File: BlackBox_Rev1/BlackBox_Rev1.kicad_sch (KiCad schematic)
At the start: 15 parts

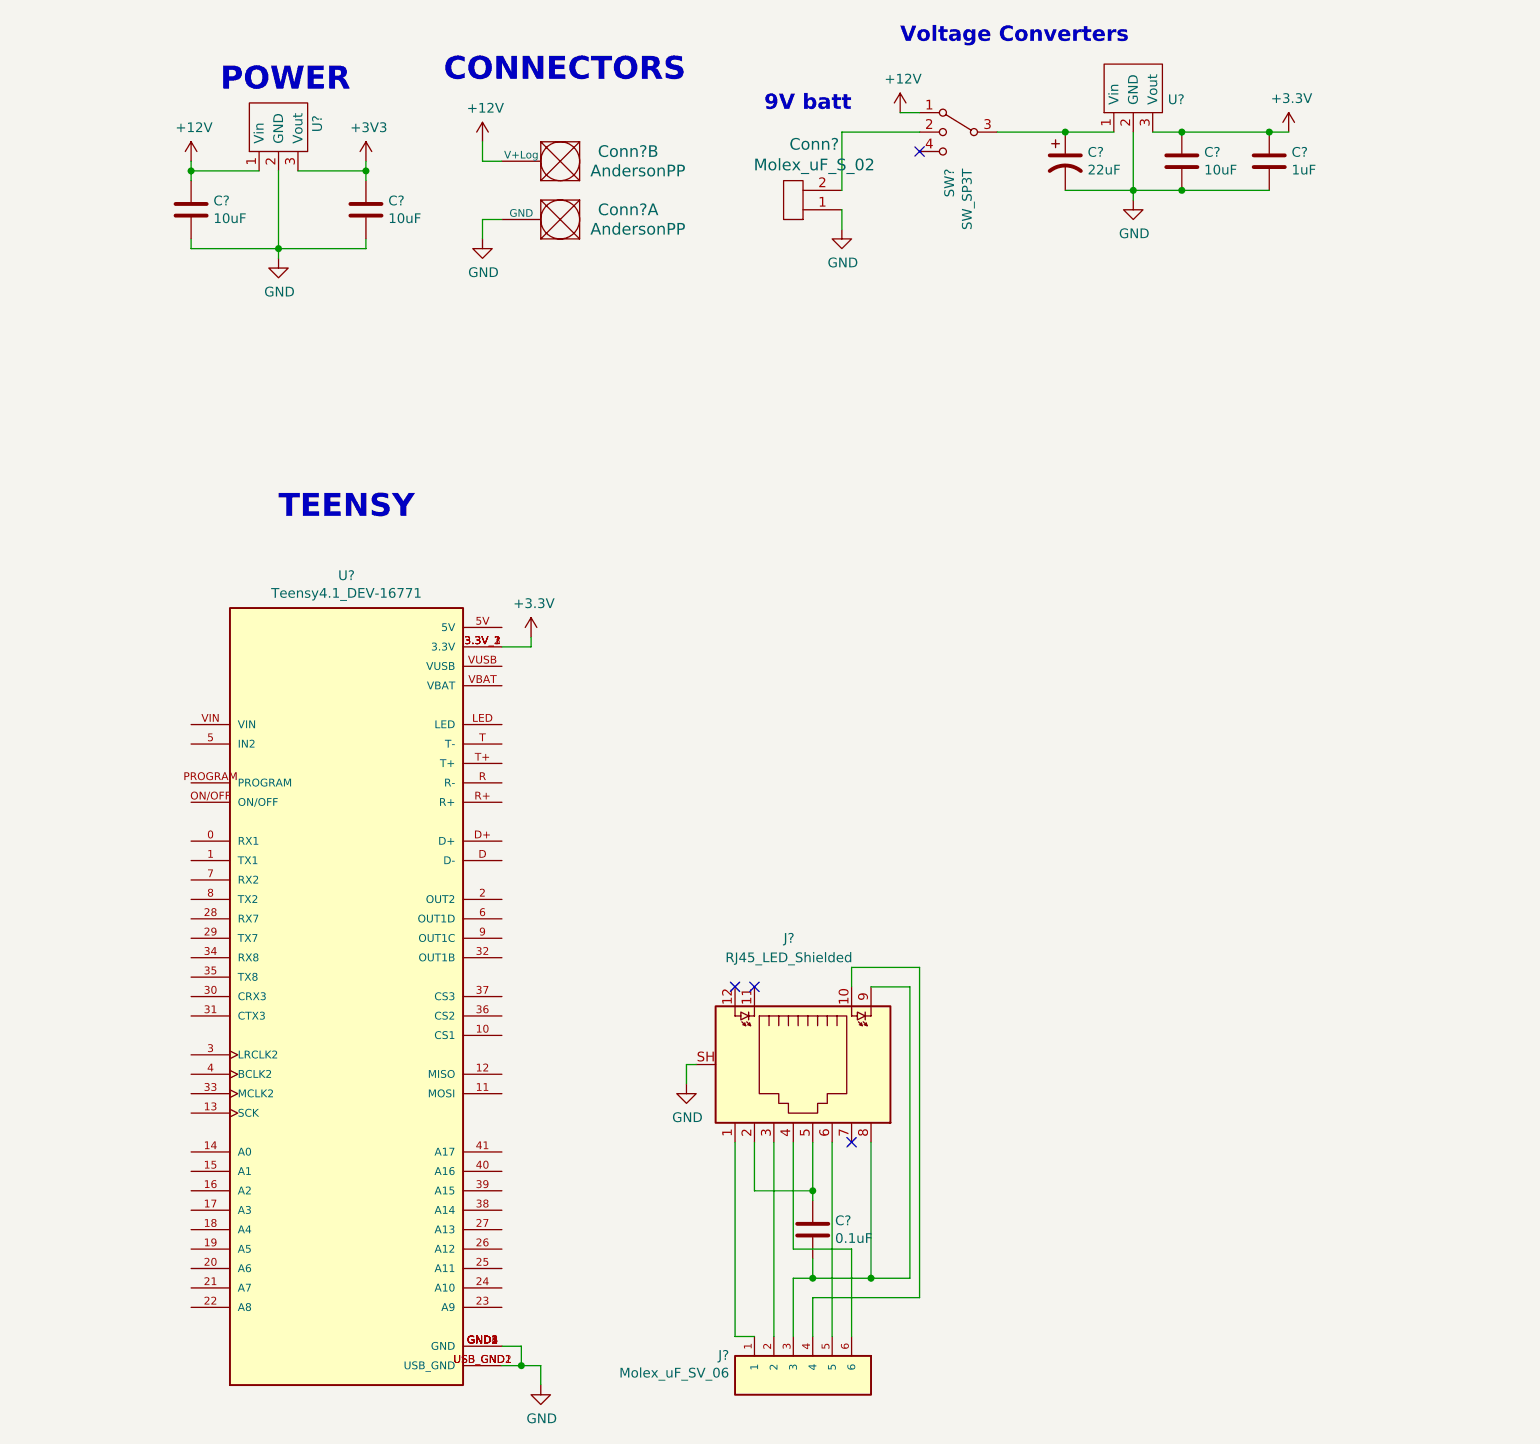
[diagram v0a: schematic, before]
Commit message: schematic design
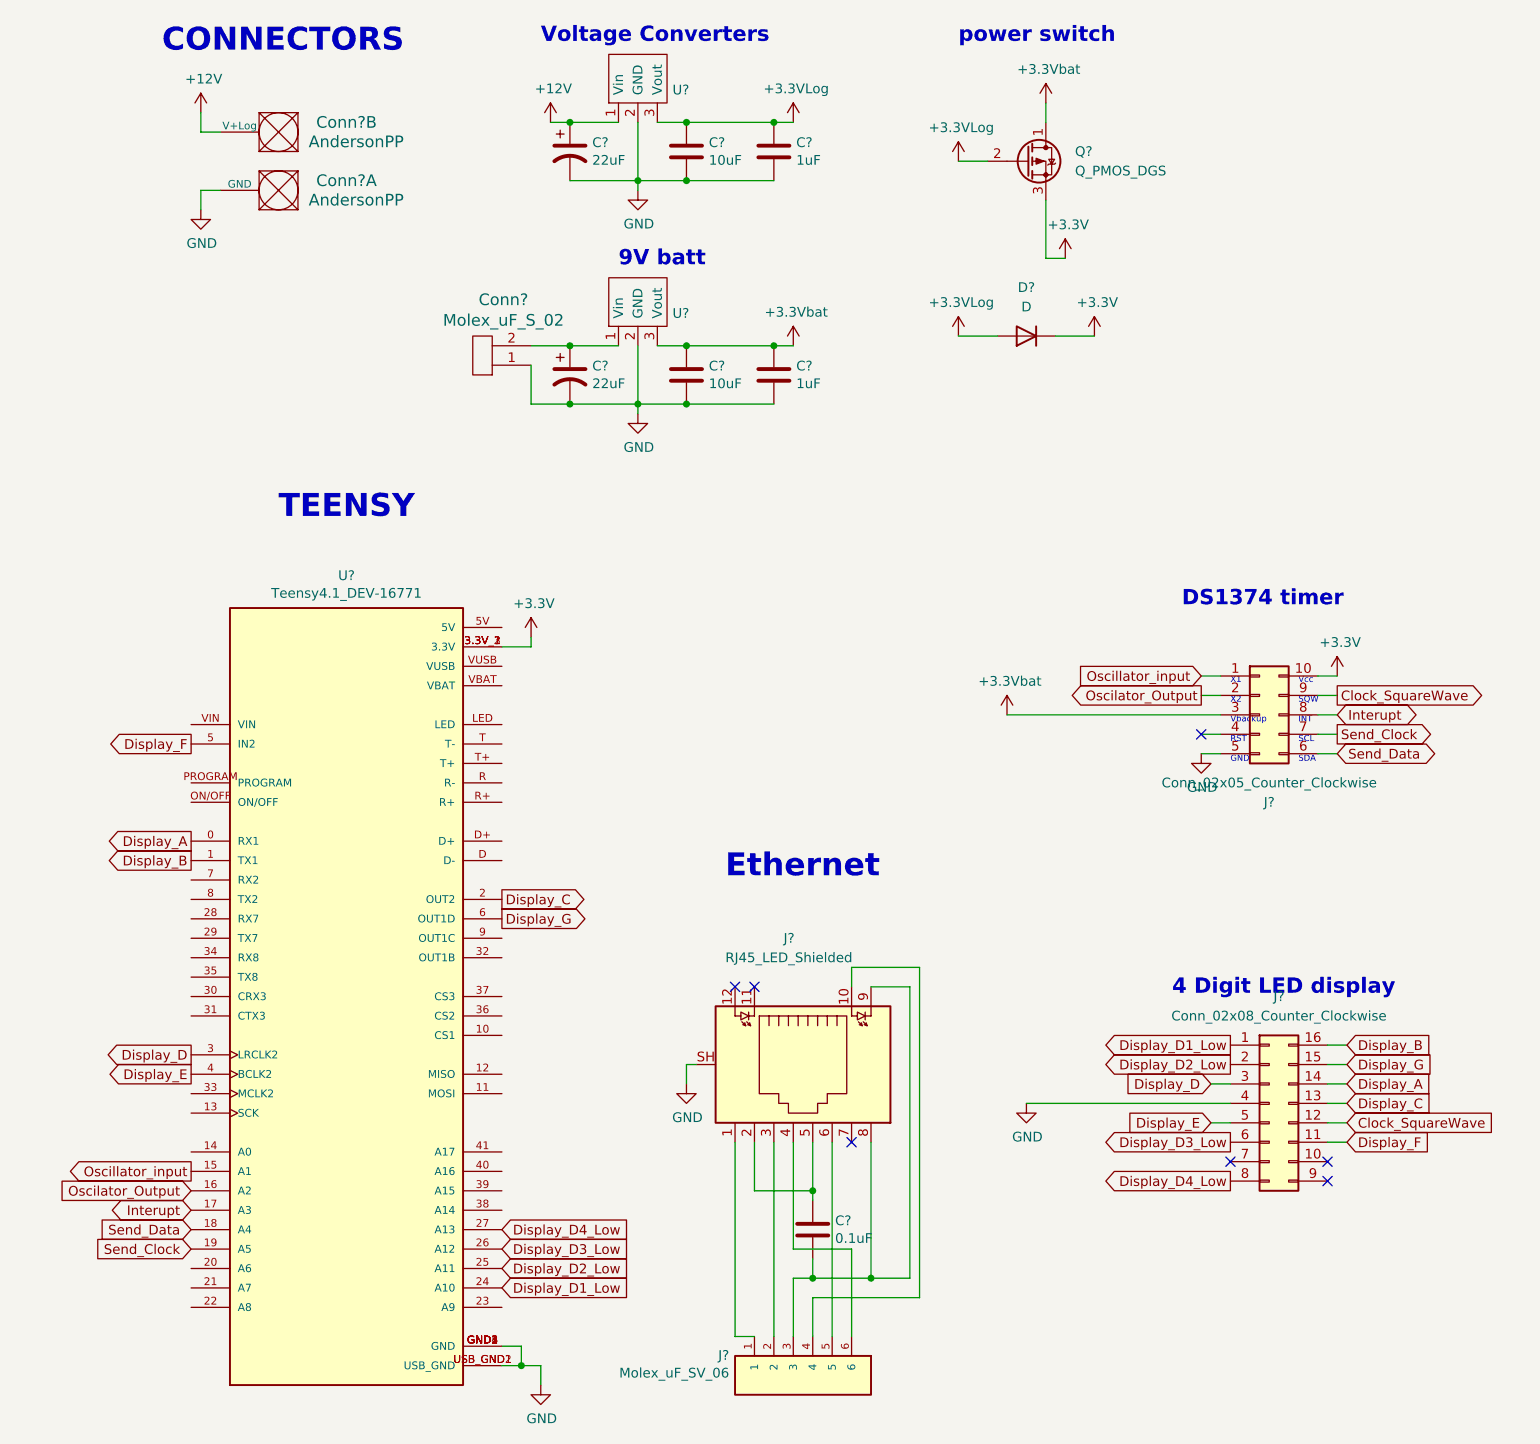
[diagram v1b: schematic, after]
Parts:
- removed C? (x2): 10uF, Capacitor_SMD:C_0603_1608Metric_Pad1.08x0.95mm_HandSolder, symbol Device:C
- removed SW?: SW_SP3T, MRDT_Connectors:MOLEX_uF_S_03_Vertical, symbol Switch:SW_SP3T
- removed U?: TSR1-2433, MRDT_Devices:TSR_1-2433, symbol Driveboard_2022-rescue:TSR1-2433-MRDT_Devices
- added C?: 1uF, Capacitor_SMD:C_0603_1608Metric_Pad1.08x0.95mm_HandSolder, symbol Device:C
- added C?: 22uF, Capacitor_THT:CP_Radial_D5.0mm_P2.00mm, symbol BMS_2022_Rev1-rescue:CP1-Device
- added C?: 10uF, Capacitor_SMD:C_0603_1608Metric_Pad1.08x0.95mm_HandSolder, symbol Device:C
- added D?: D, symbol Device:D
- added J?: Conn_02x08_Counter_Clockwise, symbol Connector_Generic:Conn_02x08_Counter_Clockwise
- added J?: Conn_02x05_Counter_Clockwise, symbol Connector_Generic:Conn_02x05_Counter_Clockwise
- added Q?: Q_PMOS_DGS, symbol Device:Q_PMOS_DGS
- added U?: TSR1-2433, MRDT_Devices:TSR_1-2433, symbol BMS_2022_Rev1-rescue:TSR1-2433-MRDT_Devices
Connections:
- net +12V: now also C?.1, U?.1 (Vin)
- net +3V3: now also C?.1, C?.1, D?.1 (K), D?.2 (A), J?.10 (Pin_10), J?.3 (Pin_3), Q?.1 (D), Q?.2 (G), Q?.3 (S), U?.3 (Vout)
- net GND: now also C?.2, C?.2, C?.2, J?.4 (Pin_4), J?.5 (Pin_5), U?.2 (GND)
- net Display_A: now reaches U?.0 (RX1)
- net Display_A: now also J?.14 (Pin_14)
- net Display_B: now reaches U?.1 (TX1)
- net Display_B: now also J?.16 (Pin_16)
- net Oscillator_input: now reaches U?.15 (A1)
- net Oscillator_input: now also J?.1 (Pin_1)
- net Oscilator_Output: now reaches U?.16 (A2)
- net Oscilator_Output: now also J?.2 (Pin_2)
- net Interupt: now reaches U?.17 (A3)
- net Interupt: now also J?.8 (Pin_8)
- net Send_Data: now reaches U?.18 (A4)
- net Send_Data: now also J?.6 (Pin_6)
- net Send_Clock: now reaches U?.19 (A5)
- net Send_Clock: now also J?.7 (Pin_7)
- net Display_C: now reaches U?.2 (OUT2)
- net Display_C: now also J?.13 (Pin_13)
- net Display_D1_Low: now reaches U?.24 (A10)
- net Display_D1_Low: now also J?.1 (Pin_1)
- net Display_D2_Low: now reaches U?.25 (A11)
- net Display_D2_Low: now also J?.2 (Pin_2)
- net Display_D3_Low: now reaches U?.26 (A12)
- net Display_D3_Low: now also J?.6 (Pin_6)
- net Display_D4_Low: now reaches U?.27 (A13)
- net Display_D4_Low: now also J?.8 (Pin_8)
- net Display_D: now reaches U?.3 (LRCLK2)
- net Display_D: now also J?.3 (Pin_3)
- net Display_E: now reaches U?.4 (BCLK2)
- net Display_E: now also J?.5 (Pin_5)
- net Display_F: now reaches U?.5 (IN2)
- net Display_F: now also J?.11 (Pin_11)
- net Display_G: now reaches U?.6 (OUT1D)
- net Display_G: now also J?.15 (Pin_15)
- net at Conn?.2: now also C?.1, U?.1 (Vin)
- new net Clock_SquareWave: J?.12 (Pin_12), J?.9 (Pin_9)
- no-connect marks 4 -> 7
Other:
- note added: "4 Digit LED display"
- note added: "DS1374 timer"
- note added: "Ethernet"
- note added: "Vcc SQW INT SCL SDA"
- note added: "X1 X2 Vbackup RST GND"
- note added: "power switch"
- note removed: "POWER"
- moved on the sheet: C?, Conn?, Conn?A, Conn?B, U?
